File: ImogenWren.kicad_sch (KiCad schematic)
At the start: 18 parts, among them J1 LiPo_4v2, J3 WS2821b, SW1 SW_SPDT_small, U1 MCP73831-2-OT

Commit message: Adding BOM
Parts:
- C1: footprint Capacitor_SMD:C_0805_2012Metric_Pad1.18x1.45mm_HandSolder -> 000_Capacitors_Immo:C_0805_2012_HandSolder_kawaii; symbol 000_Capacitor_Film_Immo:cap_film_0805 -> 000_Capacitor_Film_Immo:100n; Cost (none) -> 0.02; JLCpart (none) -> C779975
- R1, R2: symbol 000_Resistors_Immo:Resistor_0805 -> 000_Resistors_Immo:10k; Cost (none) -> 0.002; JLCpart (none) -> C2930231
- R3: symbol 000_Resistors_Immo:Resistor_0805 -> 000_Resistors_Immo:4k7; Cost (none) -> 0.002; JLCpart (none) -> C5140142
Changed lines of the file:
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@@
     )
   )
-  (symbol (lib_id "000_Resistors_Immo:Resistor_0805") (at 71.12 153.67 0) (unit 1)
+  (symbol (lib_id "000_Resistors_Immo:10k") (at 71.12 153.67 0) (unit 1)
     (in_bom yes) (on_board yes) (dnp no) (fields_autoplaced)
     (property "Reference" "R1" (at 71.12 148.59 0)
@@
       (effects (font (size 1.27 1.27)) hide)
     )
+    (property "JLCpart" "C2930231" (at 72.39 156.21 0)
+      (effects (font (size 1.27 1.27)) hide)
+    )
+    (property "Cost" "0.002" (at 71.12 156.21 0)
+      (effects (font (size 1.27 1.27)) hide)
+    )
     (pin "1")
     (pin "2")
@@
     )
   )
-  (symbol (lib_id "000_Resistors_Immo:Resistor_0805") (at 71.12 165.1 0) (unit 1)
+  (symbol (lib_id "000_Resistors_Immo:10k") (at 71.12 165.1 0) (unit 1)
     (in_bom yes) (on_board yes) (dnp no)
     (property "Reference" "R2" (at 71.12 160.02 0)
@@
     )
     (property "Datasheet" "~" (at 71.12 165.1 90)
+      (effects (font (size 1.27 1.27)) hide)
+    )
+    (property "JLCpart" "C2930231" (at 72.39 167.64 0)
+      (effects (font (size 1.27 1.27)) hide)
+    )
+    (property "Cost" "0.002" (at 71.12 167.64 0)
       (effects (font (size 1.27 1.27)) hide)
     )
@@
     )
   )
-  (symbol (lib_id "000_Capacitor_Film_Immo:cap_film_0805") (at 123.19 44.45 0) (unit 1)
+  (symbol (lib_id "000_Capacitor_Film_Immo:100n") (at 123.19 44.45 0) (unit 1)
     (in_bom yes) (on_board yes) (dnp no) (fields_autoplaced)
     (property "Reference" "C1" (at 127 43.815 0)
@@
       (effects (font (size 1.27 1.27)) (justify left))
     )
-    (property "Footprint" "Capacitor_SMD:C_0805_2012Metric_Pad1.18x1.45mm_HandSolder" (at 124.46 54.61 0)
+    (property "Footprint" "000_Capacitors_Immo:C_0805_2012_HandSolder_kawaii" (at 124.46 54.61 0)
       (effects (font (size 1.27 1.27)) hide)
     )
     (property "Datasheet" "~" (at 123.19 44.45 0)
+      (effects (font (size 1.27 1.27)) hide)
+    )
+    (property "JLCpart" "C779975" (at 124.46 54.61 0)
+      (effects (font (size 1.27 1.27)) hide)
+    )
+    (property "Cost" "0.02" (at 127 54.61 0)
       (effects (font (size 1.27 1.27)) hide)
     )
@@
     )
   )
-  (symbol (lib_id "000_Resistors_Immo:Resistor_0805") (at 71.12 177.8 0) (unit 1)
+  (symbol (lib_id "000_Resistors_Immo:4k7") (at 71.12 177.8 0) (unit 1)
     (in_bom yes) (on_board yes) (dnp no) (fields_autoplaced)
     (property "Reference" "R3" (at 71.12 172.72 0)
@@
       (effects (font (size 1.27 1.27)) hide)
     )
+    (property "JLCpart" "C5140142" (at 72.39 180.34 0)
+      (effects (font (size 1.27 1.27)) hide)
+    )
+    (property "Cost" "0.002" (at 71.12 180.34 0)
+      (effects (font (size 1.27 1.27)) hide)
+    )

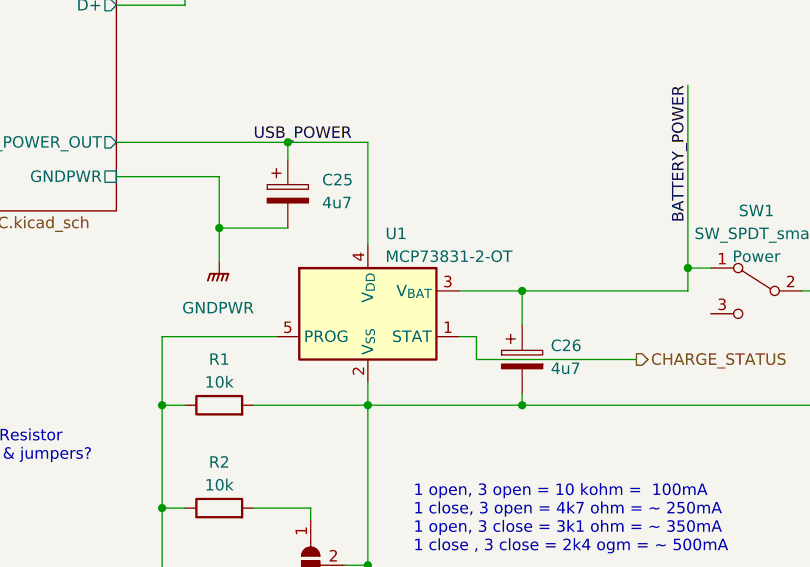
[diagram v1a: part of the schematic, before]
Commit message: dfghdfh
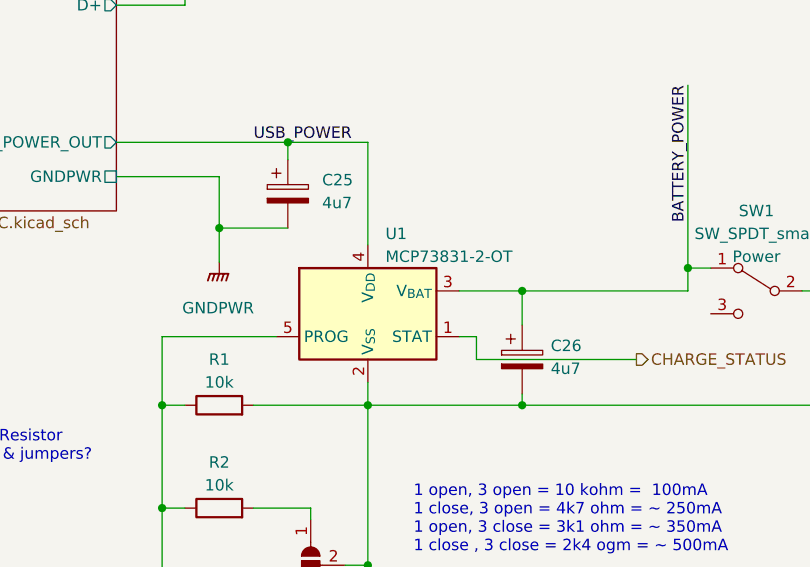
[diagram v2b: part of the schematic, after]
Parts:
- C25, C26: symbol 000_Capacitor_Film_Immo:tantalum -> 000_Capacitor_Film_Immo:4u7_tantalum; Cost (none) -> 0.0994; JLCpart (none) -> C1954175
- EC1: symbol 000_Capacitor_Electrolytic_Immo:220u -> 000_Capacitor_Electrolytic_Immo:1000uF; Cost (none) -> 0.1866; JLCpart (none) -> C134726
- R6: symbol 000_Resistors_Immo:Resistor_0805 -> 000_Resistors_Immo:470r; Cost (none) -> 0.0027; JLCpart (none) -> C280020
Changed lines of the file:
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@@
     )
   )
-  (symbol (lib_id "000_Capacitor_Electrolytic_Immo:220u") (at 181.61 36.83 0) (unit 1)
+  (symbol (lib_id "000_Capacitor_Electrolytic_Immo:1000uF") (at 181.61 36.83 0) (unit 1)
     (in_bom yes) (on_board yes) (dnp no) (fields_autoplaced)
     (property "Reference" "EC1" (at 185.42 35.306 0)
@@
       (effects (font (size 1.27 1.27)) hide)
     )
+    (property "JLCpart" "C134726" (at 181.61 36.83 0)
+      (effects (font (size 1.27 1.27)) hide)
+    )
+    (property "Cost" "0.1866" (at 181.61 36.83 0)
+      (effects (font (size 1.27 1.27)) hide)
+    )
     (pin "1")
     (pin "2")
@@
     )
   )
-  (symbol (lib_id "000_Resistors_Immo:Resistor_0805") (at 191.77 55.88 180) (unit 1)
+  (symbol (lib_id "000_Resistors_Immo:470r") (at 191.77 55.88 180) (unit 1)
     (in_bom yes) (on_board yes) (dnp no)
     (property "Reference" "R6" (at 191.77 50.8 0)
@@
     )
     (property "Datasheet" "~" (at 191.77 55.88 90)
+      (effects (font (size 1.27 1.27)) hide)
+    )
+    (property "JLCpart" "C280020" (at 190.5 53.34 0)
+      (effects (font (size 1.27 1.27)) hide)
+    )
+    (property "Cost" "0.0027" (at 191.77 53.34 0)
       (effects (font (size 1.27 1.27)) hide)
     )
@@
     )
   )
-  (symbol (lib_name "tantalum_1") (lib_id "000_Capacitor_Film_Immo:tantalum") (at 78.74 130.175 0) (unit 1)
+  (symbol (lib_id "000_Capacitor_Film_Immo:4u7_tantalum") (at 78.74 130.175 0) (unit 1)
     (in_bom yes) (on_board yes) (dnp no) (fields_autoplaced)
     (property "Reference" "C25" (at 82.55 128.651 0)
@@
     )
     (property "Datasheet" "~" (at 78.74 130.175 0)
+      (effects (font (size 1.27 1.27)) hide)
+    )
+    (property "JLCpart" "C1954175" (at 78.74 130.175 0)
+      (effects (font (size 1.27 1.27)) hide)
+    )
+    (property "Cost" "0.0994" (at 78.74 130.175 0)
       (effects (font (size 1.27 1.27)) hide)
     )
@@
     )
   )
-  (symbol (lib_id "000_Capacitor_Film_Immo:tantalum") (at 104.775 148.59 0) (unit 1)
+  (symbol (lib_id "000_Capacitor_Film_Immo:4u7_tantalum") (at 104.775 148.59 0) (unit 1)
     (in_bom yes) (on_board yes) (dnp no) (fields_autoplaced)
     (property "Reference" "C26" (at 107.95 147.066 0)
@@
       (effects (font (size 1.27 1.27)) hide)
     )
+    (property "JLCpart" "C1954175" (at 104.775 148.59 0)
+      (effects (font (size 1.27 1.27)) hide)
+    )
+    (property "Cost" "0.0994" (at 104.775 148.59 0)
+      (effects (font (size 1.27 1.27)) hide)
+    )

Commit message: dsfgdsfgd
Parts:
- SW1: Cost (none) -> 0.4487; JLCpart (none) -> C221841
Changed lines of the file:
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@@
       (effects (font (size 1.27 1.27)))
+    )
+    (property "JLCpart" "C221841" (at 130.81 140.97 0)
+      (effects (font (size 1.27 1.27)) hide)
+    )
+    (property "Cost" "0.4487" (at 130.81 140.97 0)
+      (effects (font (size 1.27 1.27)) hide)
     )
     (pin "1")
